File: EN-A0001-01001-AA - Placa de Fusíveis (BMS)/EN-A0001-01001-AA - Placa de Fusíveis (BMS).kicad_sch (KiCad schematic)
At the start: 10 parts, among them J1 INPUT, J2 OUTPUT

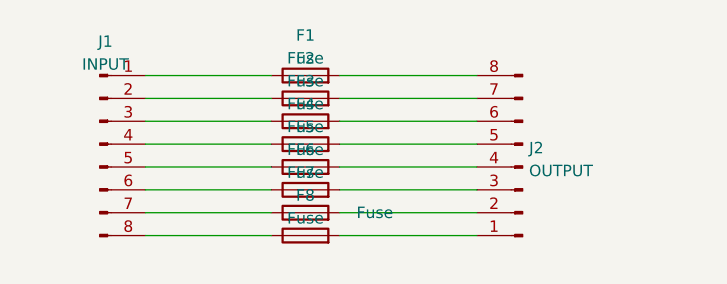
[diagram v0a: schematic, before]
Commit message: ADD: placas
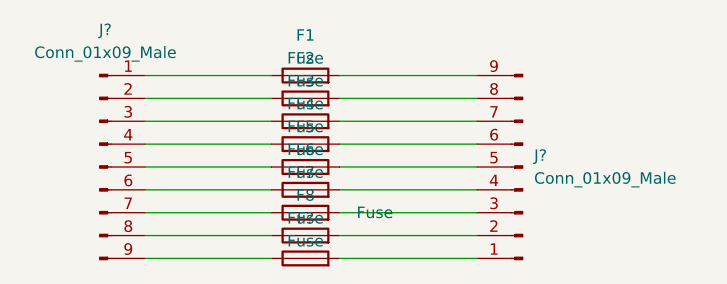
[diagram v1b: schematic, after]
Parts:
- removed J1: INPUT, Connector_PinHeader_2.54mm:PinHeader_1x08_P2.54mm_Vertical, symbol Connector:Conn_01x08_Male
- removed J2: OUTPUT, Connector_PinHeader_2.54mm:PinHeader_1x08_P2.54mm_Vertical, symbol Connector:Conn_01x08_Male
- added F?: Fuse, Fuse:Fuseholder_Cylinder-5x20mm_Schurter_0031_8201_Horizontal_Open, symbol Device:Fuse
- added J? (x2): Conn_01x09_Male, Connector_PinHeader_2.54mm:PinHeader_1x09_P2.54mm_Vertical, symbol Connector:Conn_01x09_Male
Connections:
- net at F4.1: now also J?.4 (Pin_4)
- net at F4.2: now also J?.6 (Pin_6)
- net at F7.1: now also J?.7 (Pin_7)
- net at F7.2: now also J?.3 (Pin_3)
- net at F1.1: now also J?.1 (Pin_1)
- net at F2.1: now also J?.2 (Pin_2)
- net at F3.1: now also J?.3 (Pin_3)
- net at F5.1: now also J?.5 (Pin_5)
- net at F6.1: now also J?.6 (Pin_6)
- net at F8.1: now also J?.8 (Pin_8)
- net at F8.2: now also J?.2 (Pin_2)
- net at F6.2: now also J?.4 (Pin_4)
- net at F5.2: now also J?.5 (Pin_5)
- net at F3.2: now also J?.7 (Pin_7)
- net at F2.2: now also J?.8 (Pin_8)
- net at F1.2: now also J?.9 (Pin_9)
- new net: F?.1, J?.9 (Pin_9)
- new net: F?.2, J?.1 (Pin_1)
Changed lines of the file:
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@@
+    (stroke (width 0) (type default) (color 0 0 0 0))
+  )
+  (wire (pts (xy 64.77 81.28) (xy 78.74 81.28))
     (stroke (width 0) (type default) (color 0 0 0 0))
   )
@@
   )
   (wire (pts (xy 64.77 73.66) (xy 78.74 73.66))
+    (stroke (width 0) (type default) (color 0 0 0 0))
+  )
+  (wire (pts (xy 86.36 81.28) (xy 101.6 81.28))
     (stroke (width 0) (type default) (color 0 0 0 0))
   )
@@
     (pin "2")
   )
-  (symbol (lib_id "Connector:Conn_01x08_Male") (at 59.69 68.58 0) (unit 1)
-    (in_bom yes) (on_board yes) (fields_autoplaced)
-    (property "Reference" "J1" (id 0) (at 60.325 57.184 0))
-    (property "Value" "INPUT" (id 1) (at 60.325 59.7209 0))
-    (property "Footprint" "Connector_PinHeader_2.54mm:PinHeader_1x08_P2.54mm_Vertical" (id 2) (at 59.69 68.58 0)
-      (effects (font (size 1.27 1.27)) hide)
-    )
-    (property "Datasheet" "~" (id 3) (at 59.69 68.58 0)
+  (symbol (lib_id "Device:Fuse") (at 82.55 81.28 90) (unit 1)
+    (in_bom yes) (on_board yes) (fields_autoplaced)
+    (property "Reference" "F?" (id 0) (at 82.55 76.8182 90))
+    (property "Value" "Fuse" (id 1) (at 82.55 79.3551 90))
+    (property "Footprint" "Fuse:Fuseholder_Cylinder-5x20mm_Schurter_0031_8201_Horizontal_Open" (id 2) (at 82.55 83.058 90)
+      (effects (font (size 1.27 1.27)) hide)
+    )
+    (property "Datasheet" "~" (id 3) (at 82.55 81.28 0)
+      (effects (font (size 1.27 1.27)) hide)
+    )
+    (pin "1")
+    (pin "2")
+  )
+  (symbol (lib_id "Connector:Conn_01x09_Male") (at 59.69 71.12 0) (unit 1)
+    (in_bom yes) (on_board yes) (fields_autoplaced)
+    (property "Reference" "J?" (id 0) (at 60.325 55.88 0))
+    (property "Value" "Conn_01x09_Male" (id 1) (at 60.325 58.42 0))
+    (property "Footprint" "Connector_PinHeader_2.54mm:PinHeader_1x09_P2.54mm_Vertical" (id 2) (at 59.69 71.12 0)
+      (effects (font (size 1.27 1.27)) hide)
+    )
+    (property "Datasheet" "~" (id 3) (at 59.69 71.12 0)
       (effects (font (size 1.27 1.27)) hide)
     )
@@
     (pin "7")
     (pin "8")
+    (pin "9")
   )
   (symbol (lib_id "Device:Fuse") (at 82.55 78.74 90) (unit 1)
@@
     (pin "2")
   )
-  (symbol (lib_id "Connector:Conn_01x08_Male") (at 106.68 71.12 180) (unit 1)
-    (in_bom yes) (on_board yes) (fields_autoplaced)
-    (property "Reference" "J2" (id 0) (at 107.3912 69.0153 0)
+  (symbol (lib_id "Connector:Conn_01x09_Male") (at 106.68 71.12 180) (unit 1)
+    (in_bom yes) (on_board yes) (fields_autoplaced)
+    (property "Reference" "J?" (id 0) (at 107.95 69.8499 0)
       (effects (font (size 1.27 1.27)) (justify right))
     )
-    (property "Value" "OUTPUT" (id 1) (at 107.3912 71.5522 0)
+    (property "Value" "Conn_01x09_Male" (id 1) (at 107.95 72.3899 0)
       (effects (font (size 1.27 1.27)) (justify right))
     )
-    (property "Footprint" "Connector_PinHeader_2.54mm:PinHeader_1x08_P2.54mm_Vertical" (id 2) (at 106.68 71.12 0)
+    (property "Footprint" "Connector_PinHeader_2.54mm:PinHeader_1x09_P2.54mm_Vertical" (id 2) (at 106.68 71.12 0)
       (effects (font (size 1.27 1.27)) hide)
     )
@@
     (pin "7")
     (pin "8")
+    (pin "9")
   )
   (symbol (lib_id "Device:Fuse") (at 82.55 63.5 90) (unit 1)
@@
       (reference "F8") (unit 1) (value "Fuse") (footprint "Fuse:Fuseholder_Cylinder-5x20mm_Schurter_0031_8201_Horizontal_Open")
     )
-    (path "/182fd5e7-839f-4ea9-a53f-81e4957d72db"
-      (reference "J1") (unit 1) (value "INPUT") (footprint "Connector_PinHeader_2.54mm:PinHeader_1x08_P2.54mm_Vertical")
-    )
-    (path "/85e5d25d-024a-449b-9d6c-5672650e1398"
-      (reference "J2") (unit 1) (value "OUTPUT") (footprint "Connector_PinHeader_2.54mm:PinHeader_1x08_P2.54mm_Vertical")
-    )
-  )
+    (path "/467ab26a-96c9-46b1-8c9b-3e0d54d21373"
+      (reference "F?") (unit 1) (value "Fuse") (footprint "Fuse:Fuseholder_Cylinder-5x20mm_Schurter_0031_8201_Horizontal_Open")
+    )
+    (path "/46c350bb-7de4-4e81-aafd-4af55e37aab0"
+      (reference "J?") (unit 1) (value "Conn_01x09_Male") (footprint "Connector_PinHeader_2.54mm:PinHeader_1x09_P2.54mm_Vertical")
+    )
+    (path "/63e59f98-801c-4ba0-a31f-3c2327708cfc"
+      (reference "J?") (unit 1) (value "Conn_01x09_Male") (footprint "Connector_PinHeader_2.54mm:PinHeader_1x09_P2.54mm_Vertical")
+    )
+  )
